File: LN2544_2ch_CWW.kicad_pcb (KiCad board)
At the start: 2 copper layers, 27 x 37 mm, 30 parts, among them P1 Vin, P2 LED, P3 DIM, P4 NTC, U1 LN2544, U2 LN2544

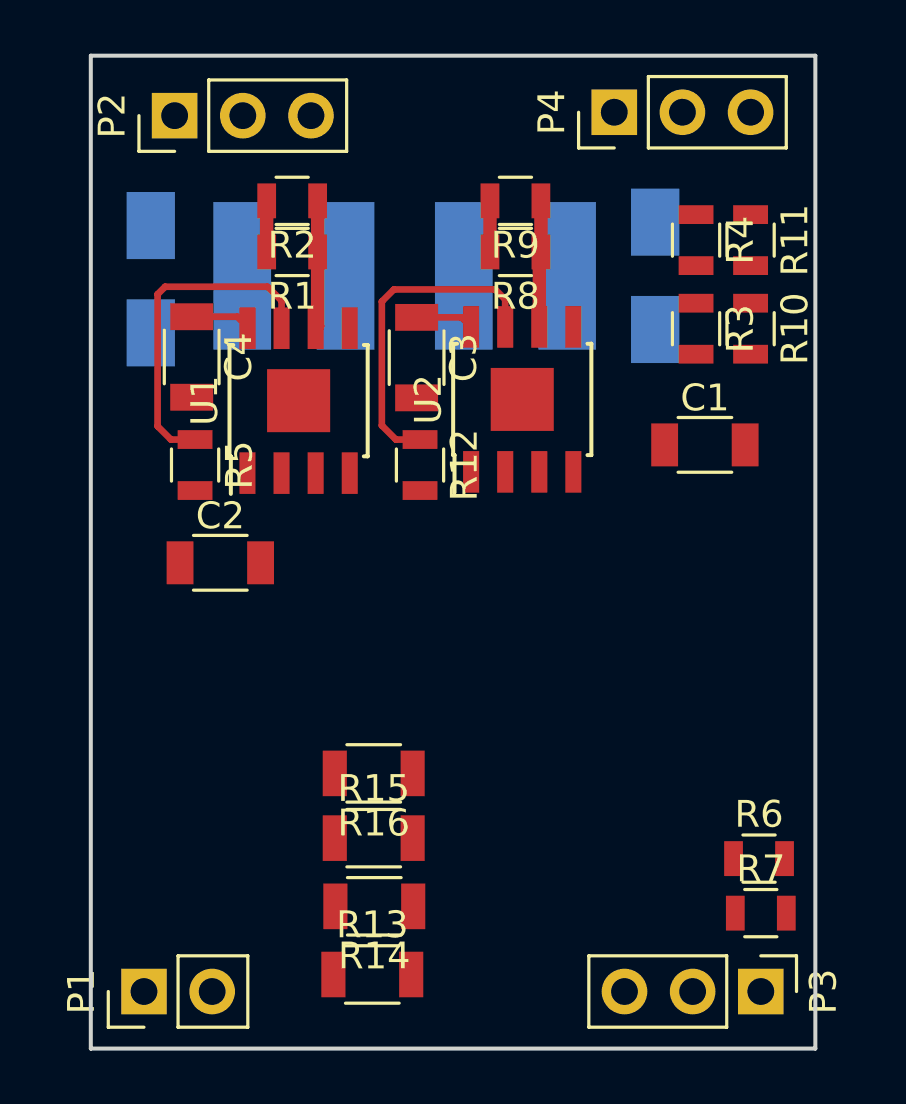
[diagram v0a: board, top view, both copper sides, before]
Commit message: PCB Update
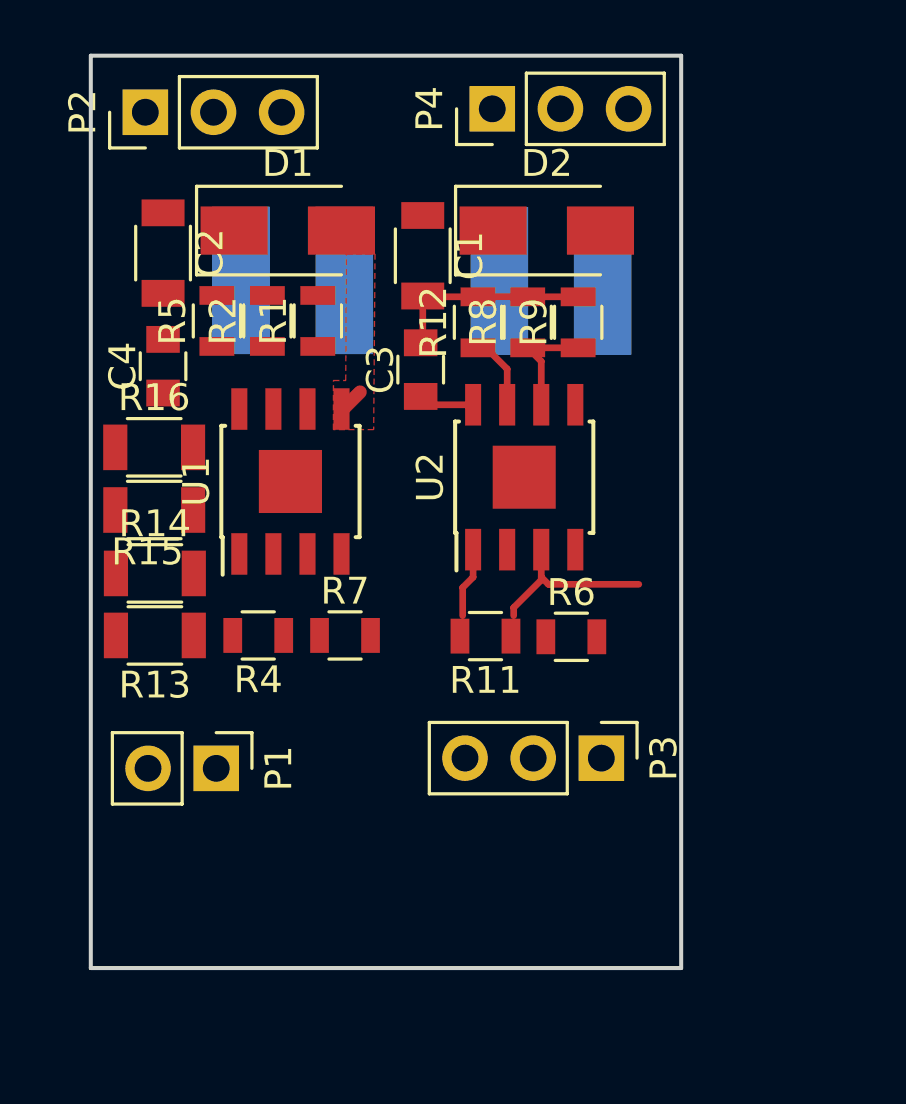
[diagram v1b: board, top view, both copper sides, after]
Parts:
- removed R10, R3: 0R, Resistors_SMD:R_0805
- C3, C4: footprint Capacitors_SMD:C_1206 -> Capacitors_SMD:C_0805
- D1, D2: moved to F.Cu
- moved R4 22.0 mm to (106.2, 121.6), turned to 180 degrees
- moved R7 18.6 mm to (109.5, 121.6)
- moved R11 17.8 mm to (114.7, 121.6), turned to 180 degrees
- moved R13 15.0 mm to (102.4, 121.6), turned to 180 degrees
- moved R14 14.9 mm to (102.4, 119.3), turned to 0 degrees
- moved R15 14.7 mm to (102.4, 116.9), turned to 180 degrees
- moved R16 14.6 mm to (102.4, 114.6), turned to 0 degrees
- moved C1 12.7 mm to (112.4, 107.5), turned to 270 degrees
- moved C2 11.7 mm to (102.7, 107.4), turned to 270 degrees
- moved R6 10.8 mm to (117.9, 121.7)
- moved P3 10.5 mm to (119.0, 126.2)
- moved P1 8.74 mm to (104.7, 126.6), turned to 270 degrees
- moved R12 5.74 mm to (114.4, 109.9), turned to 90 degrees
- moved R5 5.43 mm to (104.7, 109.9), turned to 90 degrees
- moved D1 5.42 mm to (107.3, 106.5), turned to 0 degrees
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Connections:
- P3 pad 2: /DIM1 -> /DIM2
- P3 pad 3: /DIM2 -> /DIM1
- R6 pad 1: /DIM1 -> /DIM2
- R7 pad 1: /DIM2 -> /DIM1
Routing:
- net Net-(R5-Pad1): track 12.5 -> 0.00 mm
- net Net-(R12-Pad1): track 12.2 -> 2.75 mm
- net /NTC2: track 0.00 -> 6.63 mm
- net /CS1: track 4.78 -> 0.00 mm
- net GND: track 3.81 -> 7.58 mm
- net /VREF2: track 0.00 -> 2.62 mm
- net /V_IC: track 4.47 -> 2.08 mm
- net /DRAIN1: track 0.00 -> 0.95 mm
- net /CS2: track 4.72 -> 4.21 mm
- added copper zone on F.Cu, net /DRAIN1
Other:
- board size 27 x 37 mm -> 22 x 34 mm

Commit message: PCB UPDATE
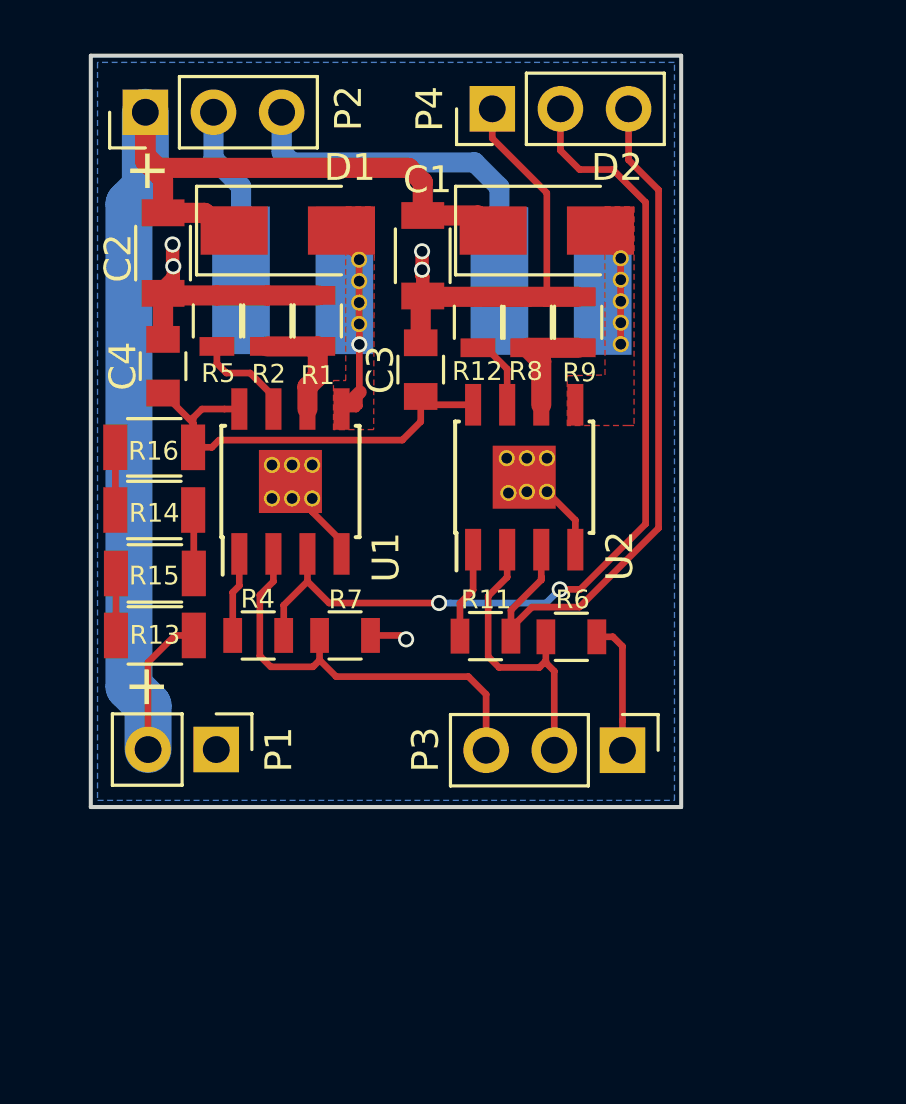
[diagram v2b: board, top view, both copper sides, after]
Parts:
- added REF**111: Via_0406, BK_Common:Via_0406, F.Cu at (115.5, 116.3)
- added REF**111: Via_0406, BK_Common:Via_0406, F.Cu at (108.2, 116.5)
- added REF**111: Via_0406, BK_Common:Via_0406, F.Cu at (108.2, 115.2)
- added REF**111: Via_0406, BK_Common:Via_0406, F.Cu at (107.5, 115.2)
- added REF**111: Via_0406, BK_Common:Via_0406, F.Cu at (110.0, 110.0)
- added REF**111: Via_0406, BK_Common:Via_0406, F.Cu at (116.2, 116.2)
- added REF**111: Via_0406, BK_Common:Via_0406, F.Cu at (117.0, 116.2)
- added REF**111: Via_0406, BK_Common:Via_0406, F.Cu at (117.0, 115.0)
- added REF**111: Via_0406, BK_Common:Via_0406, F.Cu at (116.2, 115.0)
- added REF**111: Via_0406, BK_Common:Via_0406, F.Cu at (115.5, 115.0)
- added REF**111: Via_0406, BK_Common:Via_0406, F.Cu at (106.7, 115.2)
- added REF**111: Via_0406, BK_Common:Via_0406, F.Cu at (106.7, 116.5)
- added REF**111: Via_0406, BK_Common:Via_0406, F.Cu at (107.5, 116.5)
- added REF**11111: Via_0406, BK_Common:Via_0406, F.Cu at (119.7, 110.8)
- added REF**11121: Via_0406, BK_Common:Via_0406, F.Cu at (119.7, 110.0)
- added REF**11131: Via_0406, BK_Common:Via_0406, F.Cu at (119.7, 109.2)
- added REF**11141: Via_0406, BK_Common:Via_0406, F.Cu at (119.7, 108.4)
- added REF**11151: Via_0406, BK_Common:Via_0406, F.Cu at (119.7, 107.6)
- added REF**121: Via_0406, BK_Common:Via_0406, F.Cu at (110.0, 109.2)
- added REF**131: Via_0406, BK_Common:Via_0406, F.Cu at (110.0, 108.4)
- added REF**141: Via_0406, BK_Common:Via_0406, F.Cu at (110.0, 107.6)
- moved P3 0.84 mm to (119.8, 125.9)
- moved P1 0.70 mm to (104.7, 125.9)
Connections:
- U1 pad 9: (no net) -> GND
- U2 pad 9: (no net) -> GND
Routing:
- net VCC: track 0.00 -> 53.3 mm
- net /NTC1: track 0.00 -> 35.1 mm, vias 0 -> 2
- net GND: track 7.58 -> 38.1 mm, vias 0 -> 5
- net /NTC2: track 6.63 -> 27.2 mm
- net /DIM1: track 0.00 -> 16.2 mm
- net /V_IC: track 2.08 -> 17.3 mm
- net /LEDN2: track 0.00 -> 13.6 mm
- net /DIM2: track 0.00 -> 11.1 mm
- net /DRAIN1: track 0.95 -> 8.14 mm, vias 0 -> 1
- net /LEDN1: track 0.00 -> 6.69 mm
- net /DRAIN2: track 0.00 -> 4.55 mm
- net /CS1: track 0.00 -> 4.37 mm
- net Net-(R5-Pad1): track 0.00 -> 3.72 mm
- net /VREF1: track 0.00 -> 3.14 mm
- net Net-(R14-Pad2): track 0.00 -> 2.37 mm
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- added copper zone on F.Cu, net /DRAIN2
- added copper zone on B.Cu, net GND
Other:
- board size 22 x 34 mm -> 22 x 28 mm
- rule pad_to_mask_clearance: 0.2 -> 0
- board text added: "+"
